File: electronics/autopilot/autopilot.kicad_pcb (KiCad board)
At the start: 2 copper layers, 70.4 x 68.8 mm, 27 parts, among them J1 SERVO, J10 Conn_01x03_Female, J11 Debug, J2 SERVO, J3 SERVO, J4 SERVO, J5 ESC, J6 GSM_MODULE, J7 IBUS, J8 5V IN, J9 IMU, U1 Pico, U2 SIM28ML, U3 NRF24L01_Breakout, U4 74HC244

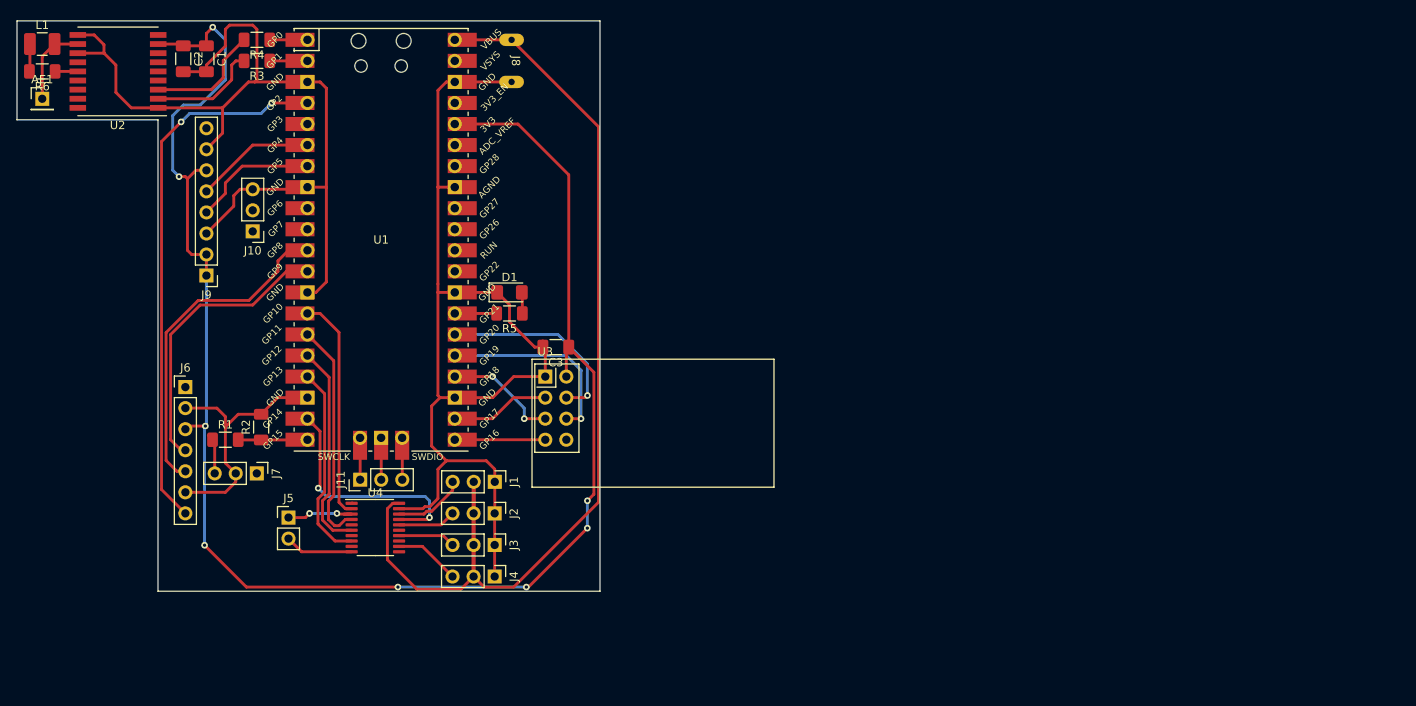
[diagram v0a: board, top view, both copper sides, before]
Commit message: minor fixes
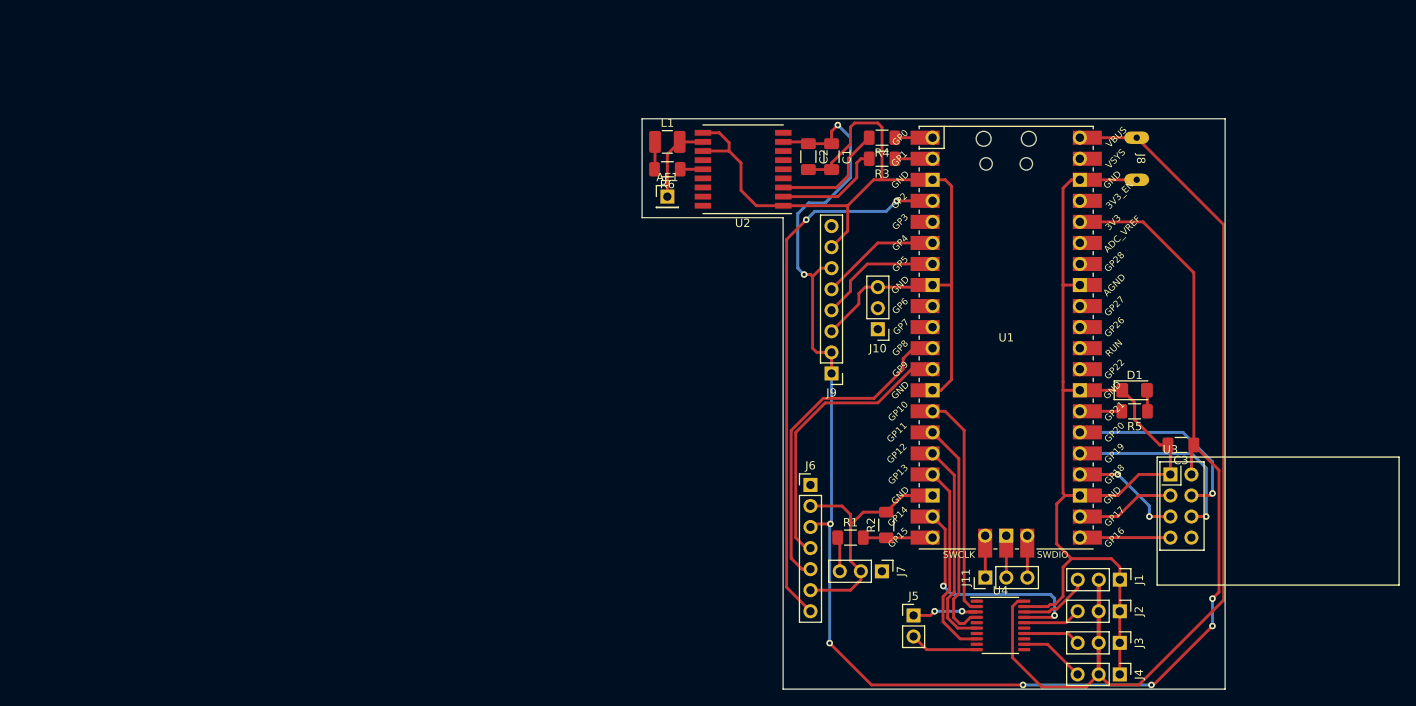
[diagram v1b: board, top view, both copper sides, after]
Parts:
- moved J5 76.4 mm to (128.3, 134.5)
- moved U3 76.4 mm to (159.3, 117.5)
- moved AE1 76.4 mm to (98.6, 83.9)
- moved C1 76.4 mm to (118.4, 79.1)
- moved D1 76.4 mm to (154.9, 107.3)
- moved J1 76.4 mm to (153.2, 130.2)
- moved J9 76.4 mm to (118.4, 105.3)
- moved L1 76.4 mm to (98.6, 77.3)
- moved R1 76.4 mm to (120.7, 125.1)
- moved R2 76.4 mm to (125.0, 123.6)
- moved R5 76.4 mm to (154.9, 109.9)
- moved R6 76.4 mm to (98.6, 80.6)
- moved U1 76.4 mm to (139.4, 101.0)
- moved C2 76.4 mm to (115.6, 79.1)
- moved C3 76.4 mm to (160.5, 113.9)
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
